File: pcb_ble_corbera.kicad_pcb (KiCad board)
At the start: 2 copper layers, 24.8 x 47.6 mm, 17 parts, among them J1 Conn_01x02, J2 Conn_02x04_Odd_Even, J4 Conn_ARM_JTAG_SWD_10, SW1 SW_Push, U1 BL652, U2 HDC1080

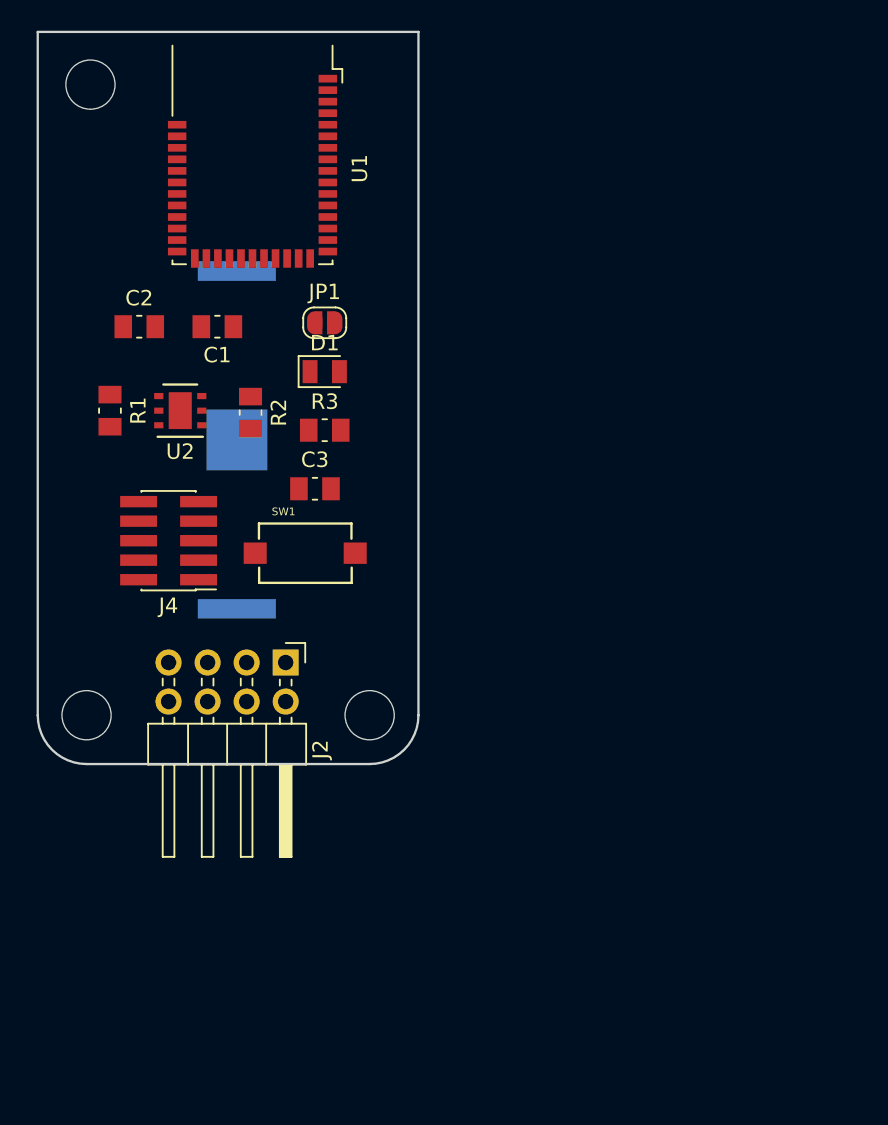
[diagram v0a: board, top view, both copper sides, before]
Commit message: new tracks
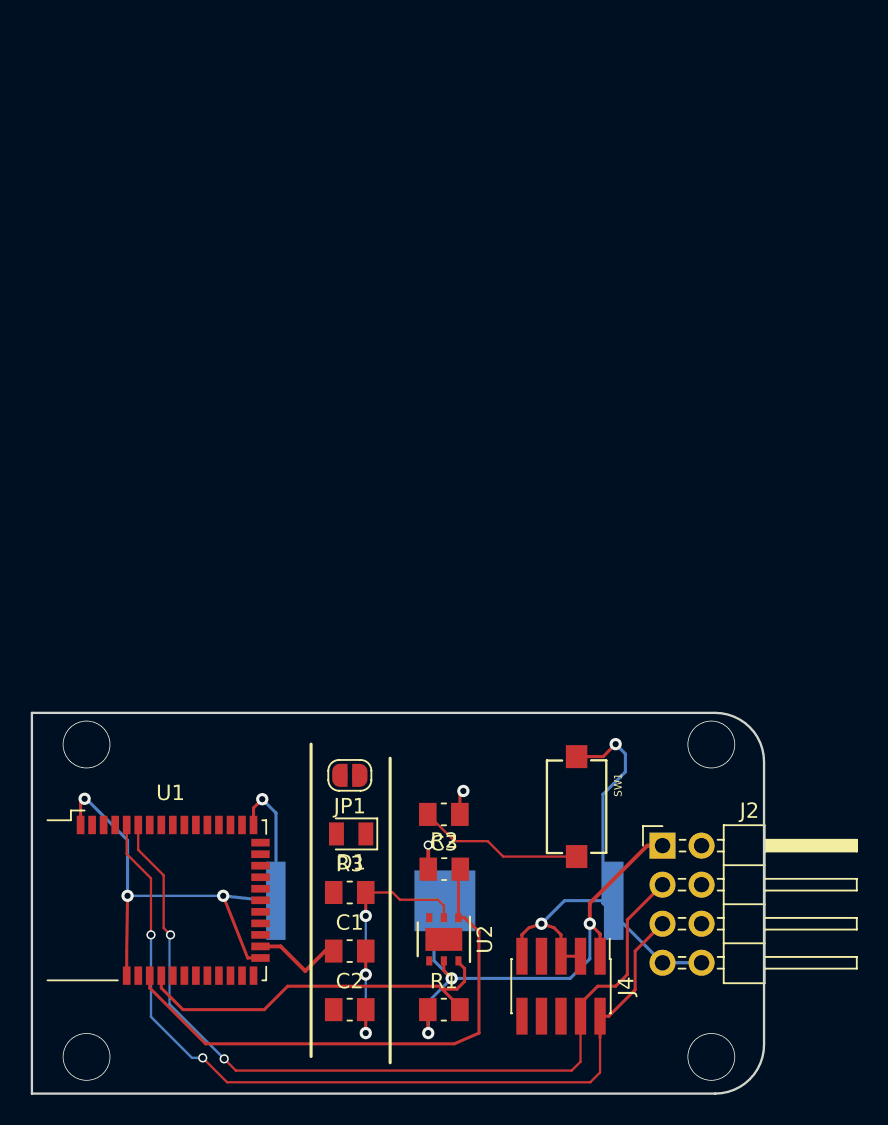
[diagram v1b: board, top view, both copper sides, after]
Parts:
- removed REF** (x3): MountingHole_3.2mm_M3_DIN965, MountingHole:MountingHole_3.2mm_M3_DIN965
- moved U1 47.9 mm to (138.8, 95.2), turned to 0 degrees
- moved C2 46.5 mm to (150.5, 102.3)
- moved R1 44.6 mm to (156.6, 102.3), turned to 0 degrees
- moved C1 41.5 mm to (150.5, 98.5), turned to 0 degrees
- moved J4 38.6 mm to (164.2, 100.8), turned to 270 degrees
- moved U2 38.4 mm to (156.6, 97.8), turned to 270 degrees
- moved J1 32.9 mm to (156.7, 95.2), turned to 180 degrees
- moved R2 32.3 mm to (156.6, 93.2), turned to 0 degrees
- moved D1 30.1 mm to (150.6, 90.9), turned to 180 degrees
- moved R3 30.1 mm to (150.5, 94.7)
- moved JP1 29.5 mm to (150.5, 87.1), turned to 0 degrees
- moved J2 27.3 mm to (170.8, 91.7), turned to 0 degrees
- moved SW1 24.2 mm to (165.2, 89.1), turned to 270 degrees
- moved C3 22.8 mm to (156.6, 89.6), turned to 0 degrees
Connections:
- J2 pad 4: SERIAL_RX -> SERIAL_TX
- U1 pad 17: SERIAL_RX -> SERIAL_TX
- U2 pad 7: GND -> Net-(U2-Pad7)
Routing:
- net GND: track 0.00 -> 92.1 mm, vias 0 -> 10
- net SWDIO-TMS: track 0.00 -> 57.5 mm, vias 0 -> 2
- net SWDCLK: track 0.00 -> 55.7 mm, vias 0 -> 2
- net VCC: track 0.00 -> 42.3 mm, vias 0 -> 4
- net SDA: track 0.00 -> 35.4 mm
- net SCL: track 0.00 -> 25.6 mm
- net BUTTON_0: track 0.00 -> 11.0 mm
- net (no net): vias 0 -> 4
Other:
- board size 24.8 x 47.6 mm -> 47.6 x 24.8 mm
- net class Default: trace_width 0.2 -> 0.1524; via_dia 0.8 -> 0.6
- net class Power: clearance 0.15 -> 0.25; trace_width 0.15 -> 0.254
